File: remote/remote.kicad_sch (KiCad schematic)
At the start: 26 parts, among them J1 USB-C, SW1 Choc1, SW2 Choc2, U1 ESP32-C3-WROOM-02, U2 MCP73831, U3 AP2112K-3.3

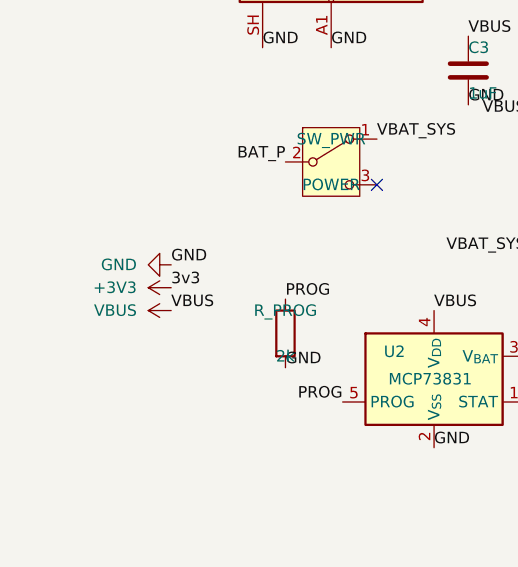
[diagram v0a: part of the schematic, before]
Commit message: fix stuff
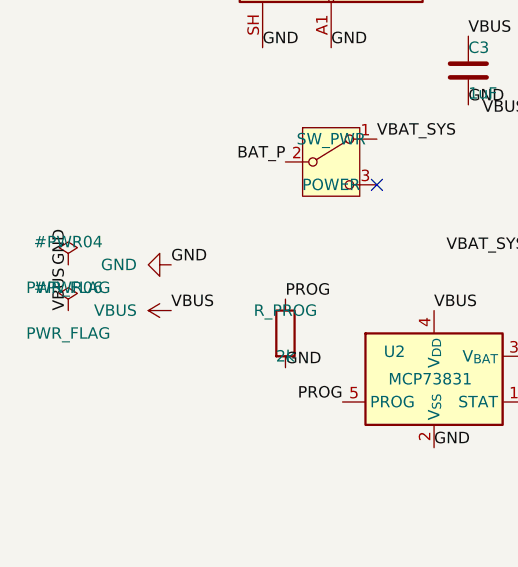
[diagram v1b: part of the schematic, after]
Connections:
- net +3V3 renamed 3v3
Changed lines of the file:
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@@
-		)
-	)
-	(label "3v3"
-		(at 26.67 119.38 0)
-		(effects
-			(font
-				(size 1.27 1.27)
-			)
-			(justify left bottom)
 		)
 	)
@@
 	)
 	(symbol
-		(lib_id "power:+3V3")
-		(at 26.67 119.38 90)
-		(unit 1)
-		(body_style 1)
-		(exclude_from_sim no)
-		(in_bom yes)
-		(on_board yes)
-		(in_pos_files yes)
-		(dnp no)
-		(fields_autoplaced yes)
-		(property "Reference" "#PWR02"
-			(at 30.48 119.38 0)
-			(hide yes)
-			(show_name no)
-			(do_not_autoplace no)
-			(effects
-				(font
-					(size 1.27 1.27)
-				)
-			)
-		)
-		(property "Value" "+3V3"
-			(at 22.86 119.3799 90)
-			(show_name no)
-			(do_not_autoplace no)
-			(effects
-				(font
-					(size 1.27 1.27)
-				)
-				(justify left)
-			)
-		)
-		(property "Footprint" ""
-			(at 26.67 119.38 0)
-			(hide yes)
-			(show_name no)
-			(do_not_autoplace no)
-			(effects
-				(font
-					(size 1.27 1.27)
-				)
-			)
-		)
-		(property "Datasheet" ""
-			(at 26.67 119.38 0)
-			(hide yes)
-			(show_name no)
-			(do_not_autoplace no)
-			(effects
-				(font
-					(size 1.27 1.27)
-				)
-			)
-		)
-		(property "Description" "Power symbol creates a global label with name \"+3V3\""
-			(at 26.67 119.38 0)
-			(hide yes)
-			(show_name no)
-			(do_not_autoplace no)
-			(effects
-				(font
-					(size 1.27 1.27)
-				)
-			)
-		)
-		(pin "1"
-		)
-		(instances
-			(project "remote"
-				(path "/0f8715e9-9989-48cf-8f39-458c5e68edc6"
-					(reference "#PWR02")
-					(unit 1)
-				)
-			)
-		)
-	)
-	(symbol
 		(lib_id "Device:R")
 		(at 76.2 58.42 0)
@@
 		)
 	)
+	(symbol
+		(lib_id "power:PWR_FLAG")
+		(at 15.24 116.84 0)
+		(unit 1)
+		(body_style 1)
+		(exclude_from_sim no)
+		(in_bom yes)
+		(on_board yes)
+		(in_pos_files yes)
+		(dnp no)
+		(property "Reference" "#PWR04"
+			(at 15.24 114.3 0)
+			(show_name no)
+			(do_not_autoplace no)
+			(effects
+				(font
+					(size 1.27 1.27)
+				)
+			)
+		)
+		(property "Value" "PWR_FLAG"
+			(at 15.24 119.38 0)
+			(show_name no)
+			(do_not_autoplace no)
+			(effects
+				(font
+					(size 1.27 1.27)
+				)
+			)
+		)
+		(property "Footprint" ""
+			(at 15.24 116.84 0)
+			(hide yes)
+			(show_name no)
+			(do_not_autoplace no)
+			(effects
+				(font
+					(size 1.27 1.27)
+				)
+			)
+		)
+		(property "Datasheet" ""
+			(at 15.24 116.84 0)
+			(hide yes)
+			(show_name no)
+			(do_not_autoplace no)
+			(effects
+				(font
+					(size 1.27 1.27)
+				)
+			)
+		)
+		(property "Description" "Special symbol for telling ERC where power comes from"
+			(at 15.24 116.84 0)
+			(hide yes)
+			(show_name no)
+			(do_not_autoplace no)
+			(effects
+				(font
+					(size 1.27 1.27)
+				)
+			)
+		)
+		(pin "1"
+		)
+		(instances
+			(project "remote"
+				(path "/0f8715e9-9989-48cf-8f39-458c5e68edc6"
+					(reference "#PWR04")
+					(unit 1)
+				)
+			)
+		)
+	)
+	(symbol
+		(lib_id "power:PWR_FLAG")
+		(at 15.24 121.92 0)
+		(unit 1)
+		(body_style 1)
+		(exclude_from_sim no)
+		(in_bom yes)
+		(on_board yes)
+		(in_pos_files yes)
+		(dnp no)
+		(property "Reference" "#PWR06"
+			(at 15.24 119.38 0)
+			(show_name no)
+			(do_not_autoplace no)
+			(effects
+				(font
+					(size 1.27 1.27)
+				)
+			)
+		)
+		(property "Value" "PWR_FLAG"
+			(at 15.24 124.46 0)
+			(show_name no)
+			(do_not_autoplace no)
+			(effects
+				(font
+					(size 1.27 1.27)
+				)
+			)
+		)
+		(property "Footprint" ""
+			(at 15.24 121.92 0)
+			(hide yes)
+			(show_name no)
+			(do_not_autoplace no)
+			(effects
+				(font
+					(size 1.27 1.27)
+				)
+			)
+		)
+		(property "Datasheet" ""
+			(at 15.24 121.92 0)
+			(hide yes)
+			(show_name no)
+			(do_not_autoplace no)
+			(effects
+				(font
+					(size 1.27 1.27)
+				)
+			)
+		)
+		(property "Description" "Special symbol for telling ERC where power comes from"
+			(at 15.24 121.92 0)
+			(hide yes)
+			(show_name no)
+			(do_not_autoplace no)
+			(effects
+				(font
+					(size 1.27 1.27)
+				)
+			)
+		)
+		(pin "1"
+		)
+		(instances
+			(project "remote"
+				(path "/0f8715e9-9989-48cf-8f39-458c5e68edc6"
+					(reference "#PWR06")
+					(unit 1)
+				)
+			)
+		)
+	)
+	(label "GND"
+		(at 15.24 116.84 90)
+		(effects
+			(font
+				(size 1.27 1.27)
+			)
+			(justify left bottom)
+		)
+	)
+	(label "VBUS"
+		(at 15.24 121.92 90)
+		(effects
+			(font
+				(size 1.27 1.27)
+			)
+			(justify left bottom)
+		)
+	)

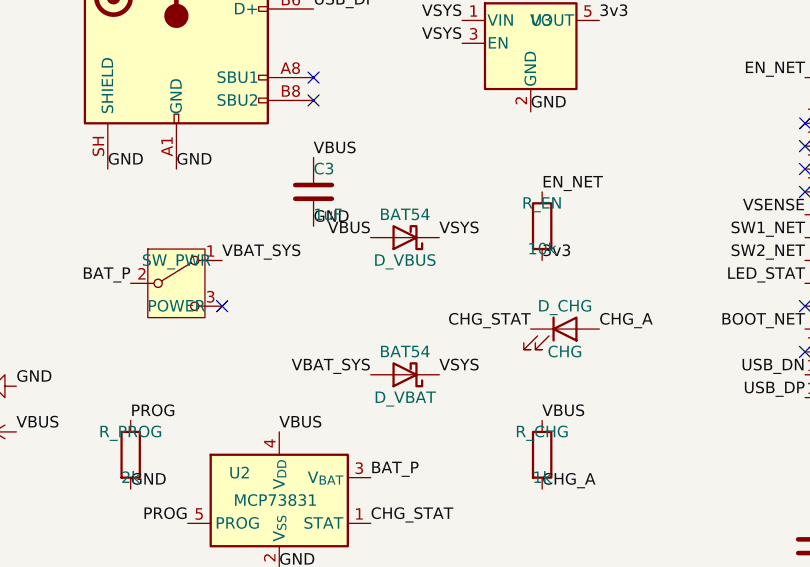
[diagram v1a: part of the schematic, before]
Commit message: devlog 04
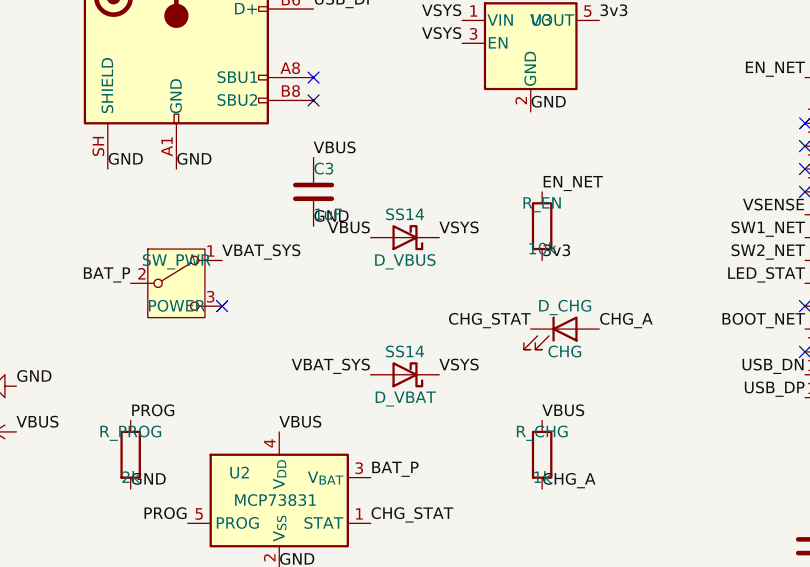
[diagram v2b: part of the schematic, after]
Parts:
- C1, C2, C3: footprint (none) -> Capacitor_SMD:C_0603_1608Metric
- D_CHG, D_STAT: footprint (none) -> LED_SMD:LED_0603_1608Metric
- D_VBAT, D_VBUS: value BAT54 -> SS14; footprint (none) -> Diode_SMD:D_SMA
- HDR1: footprint (none) -> Connector_PinHeader_2.54mm:PinHeader_1x03_P2.54mm_Vertical
- J1: footprint (none) -> Connector_USB:USB_C_Receptacle_HRO_TYPE-C-31-M-12
- J_BAT: footprint (none) -> Connector_JST:JST_PH_B2B-PH-K_1x02_P2.00mm_Vertical
- R_CC1, R_CC2, R_CHG, R_DN, R_EN, R_PROG, R_STAT, R_UP: footprint (none) -> Resistor_SMD:R_0603_1608Metric
- SW1, SW2: footprint (none) -> clicker:Choc_V1_PG1350
- SW_BOOT, SW_RST: footprint (none) -> Button_Switch_SMD:SW_SPST_B3U-1000P
- SW_PWR: footprint (none) -> Button_Switch_THT:SW_Slide_SPDT_Straight_CK_OS102011MS2Q
- U1: footprint (none) -> RF_Module:ESP32-C3-WROOM-02
- U2, U3: footprint (none) -> Package_TO_SOT_SMD:SOT-23-5
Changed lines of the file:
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@@
 			)
 		)
-		(property "Footprint" ""
+		(property "Footprint" "Button_Switch_THT:SW_Slide_SPDT_Straight_CK_OS102011MS2Q"
 			(at 44.45 105.41 0)
 			(hide yes)
@@
 			)
 		)
-		(property "Footprint" ""
+		(property "Footprint" "Resistor_SMD:R_0603_1608Metric"
 			(at 127.762 165.1 90)
 			(hide yes)
@@
 			)
 		)
-		(property "Footprint" ""
+		(property "Footprint" "RF_Module:ESP32-C3-WROOM-02"
 			(at 129.54 100.965 0)
 			(hide yes)
@@
 			)
 		)
-		(property "Footprint" ""
+		(property "Footprint" "Package_TO_SOT_SMD:SOT-23-5"
 			(at 83.82 86.995 0)
 			(hide yes)
@@
 			)
 		)
-		(property "Footprint" ""
+		(property "Footprint" "Capacitor_SMD:C_0603_1608Metric"
 			(at 130.505 130.81 0)
 			(hide yes)
@@
 			)
 		)
-		(property "Footprint" ""
+		(property "Footprint" "Resistor_SMD:R_0603_1608Metric"
 			(at 83.312 99.06 90)
 			(hide yes)
@@
 			)
 		)
-		(property "Footprint" ""
+		(property "Footprint" "clicker:Choc_V1_PG1350"
 			(at 185.42 120.65 0)
 			(hide yes)
@@
 			)
 		)
-		(property "Footprint" ""
+		(property "Footprint" "clicker:Choc_V1_PG1350"
 			(at 185.42 80.01 0)
 			(hide yes)
@@
 			)
 		)
-		(property "Value" "BAT54"
+		(property "Value" "SS14"
 			(at 69.85 97.79 0)
 			(show_name no)
@@
 			)
 		)
-		(property "Footprint" ""
+		(property "Footprint" "Diode_SMD:D_SMA"
 			(at 69.85 100.33 0)
 			(hide yes)
@@
 			)
 		)
-		(property "Footprint" ""
+		(property "Footprint" "Button_Switch_SMD:SW_SPST_B3U-1000P"
 			(at 175.26 160.02 0)
 			(hide yes)
@@
 			)
 		)
-		(property "Footprint" ""
+		(property "Footprint" "Resistor_SMD:R_0603_1608Metric"
 			(at 88.392 154.94 90)
 			(hide yes)
@@
 			)
 		)
-		(property "Footprint" ""
+		(property "Footprint" "Resistor_SMD:R_0603_1608Metric"
 			(at 37.592 124.46 90)
 			(hide yes)
@@
 			)
 		)
-		(property "Footprint" ""
+		(property "Footprint" "Package_TO_SOT_SMD:SOT-23-5"
 			(at 57.15 123.19 0)
 			(hide yes)
@@
 			)
 		)
-		(property "Footprint" ""
+		(property "Footprint" "Resistor_SMD:R_0603_1608Metric"
 			(at 74.422 46.99 90)
 			(hide yes)
@@
 			)
 		)
-		(property "Footprint" ""
+		(property "Footprint" "Connector_PinHeader_2.54mm:PinHeader_1x03_P2.54mm_Vertical"
 			(at 165.1 99.06 0)
 			(hide yes)
@@
 			)
 		)
-		(property "Value" "BAT54"
+		(property "Value" "SS14"
 			(at 69.85 113.03 0)
 			(show_name no)
@@
 			)
 		)
-		(property "Footprint" ""
+		(property "Footprint" "Diode_SMD:D_SMA"
 			(at 69.85 115.57 0)
 			(hide yes)
@@
 			)
 		)
-		(property "Footprint" ""
+		(property "Footprint" "LED_SMD:LED_0603_1608Metric"
 			(at 129.54 149.86 0)
 			(hide yes)
@@
 			)
 		)
-		(property "Footprint" ""
+		(property "Footprint" "Connector_USB:USB_C_Receptacle_HRO_TYPE-C-31-M-12"
 			(at 48.26 69.85 0)
 			(hide yes)
@@
 			)
 		)
-		(property "Footprint" ""
+		(property "Footprint" "Resistor_SMD:R_0603_1608Metric"
 			(at 83.312 124.46 90)
 			(hide yes)
@@
 			)
 		)
-		(property "Footprint" ""
+		(property "Footprint" "Connector_JST:JST_PH_B2B-PH-K_1x02_P2.00mm_Vertical"
 			(at 39.37 154.94 0)
 			(hide yes)
@@
 			)
 		)
-		(property "Footprint" ""
+		(property "Footprint" "Capacitor_SMD:C_0603_1608Metric"
 			(at 60.655 91.44 0)
 			(hide yes)
@@
 			)
 		)
-		(property "Footprint" ""
+		(property "Footprint" "Button_Switch_SMD:SW_SPST_B3U-1000P"
 			(at 154.94 160.02 0)
 			(hide yes)
@@
 			)
 		)
-		(property "Footprint" ""
+		(property "Footprint" "Resistor_SMD:R_0603_1608Metric"
 			(at 74.422 58.42 90)
 			(hide yes)
@@
 			)
 		)
-		(property "Footprint" ""
+		(property "Footprint" "LED_SMD:LED_0603_1608Metric"
 			(at 87.63 110.49 0)
 			(hide yes)
@@
 			)
 		)
-		(property "Footprint" ""
+		(property "Footprint" "Capacitor_SMD:C_0603_1608Metric"
 			(at 116.535 130.81 0)
 			(hide yes)
@@
 			)
 		)
-		(property "Footprint" ""
+		(property "Footprint" "Resistor_SMD:R_0603_1608Metric"
 			(at 103.632 154.94 90)
 			(hide yes)

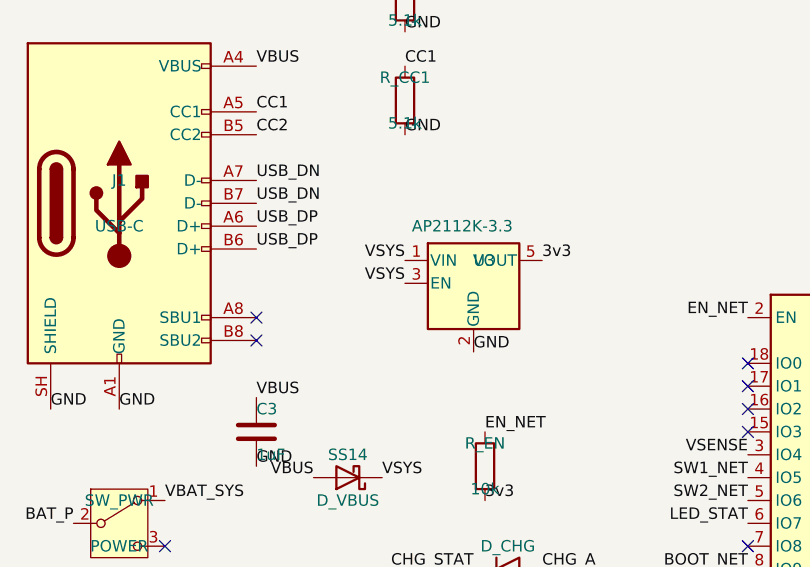
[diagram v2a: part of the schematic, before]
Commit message: devlog 08
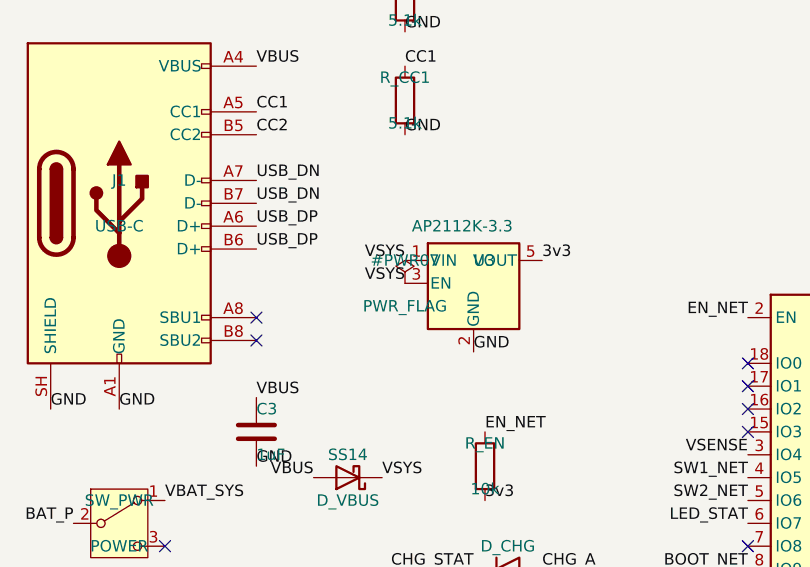
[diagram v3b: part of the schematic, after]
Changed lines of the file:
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@@
+	(symbol
+		(lib_id "power:PWR_FLAG")
+		(at 76.2 78.74 0)
+		(unit 1)
+		(body_style 1)
+		(exclude_from_sim no)
+		(in_bom yes)
+		(on_board yes)
+		(in_pos_files yes)
+		(dnp no)
+		(property "Reference" "#PWR07"
+			(at 76.2 76.2 0)
+			(show_name no)
+			(do_not_autoplace no)
+			(effects
+				(font
+					(size 1.27 1.27)
+				)
+			)
+		)
+		(property "Value" "PWR_FLAG"
+			(at 76.2 81.28 0)
+			(show_name no)
+			(do_not_autoplace no)
+			(effects
+				(font
+					(size 1.27 1.27)
+				)
+			)
+		)
+		(property "Footprint" ""
+			(at 76.2 78.74 0)
+			(hide yes)
+			(show_name no)
+			(do_not_autoplace no)
+			(effects
+				(font
+					(size 1.27 1.27)
+				)
+			)
+		)
+		(property "Datasheet" ""
+			(at 76.2 78.74 0)
+			(hide yes)
+			(show_name no)
+			(do_not_autoplace no)
+			(effects
+				(font
+					(size 1.27 1.27)
+				)
+			)
+		)
+		(property "Description" "Special symbol for telling ERC where power comes from"
+			(at 76.2 78.74 0)
+			(hide yes)
+			(show_name no)
+			(do_not_autoplace no)
+			(effects
+				(font
+					(size 1.27 1.27)
+				)
+			)
+		)
+		(pin "1"
+		)
+		(instances
+			(project "remote"
+				(path "/0f8715e9-9989-48cf-8f39-458c5e68edc6"
+					(reference "#PWR07")
+					(unit 1)
+				)
+			)
+		)
+	)
 	(symbol
 		(lib_id "power:PWR_FLAG")
